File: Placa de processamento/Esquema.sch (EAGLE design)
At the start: 14 parts

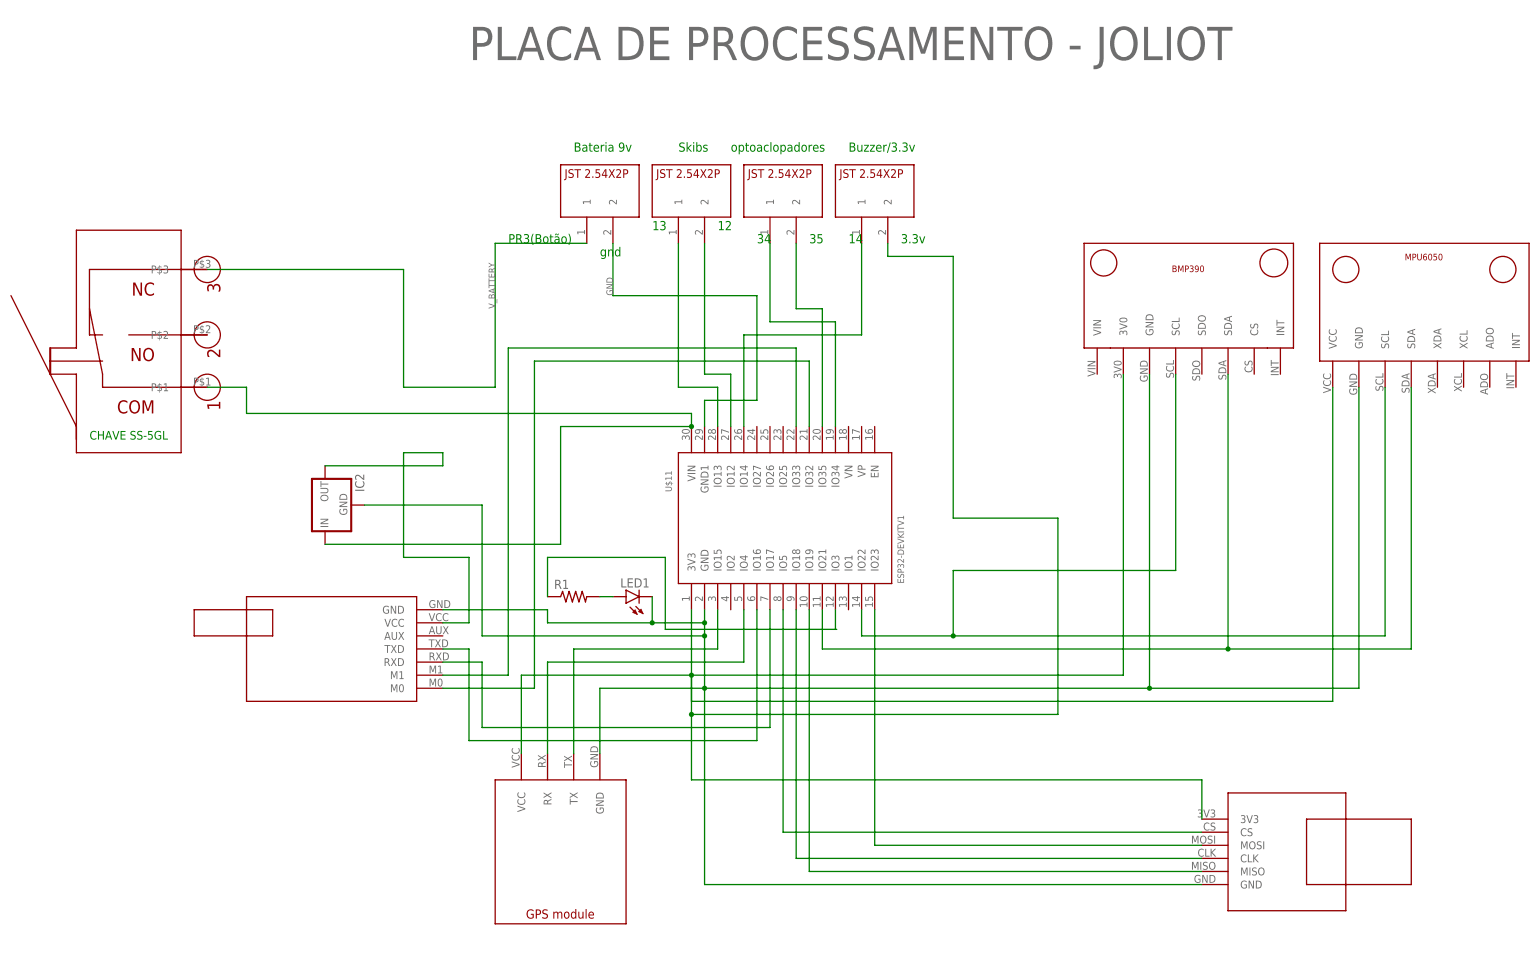
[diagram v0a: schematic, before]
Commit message: Coisas
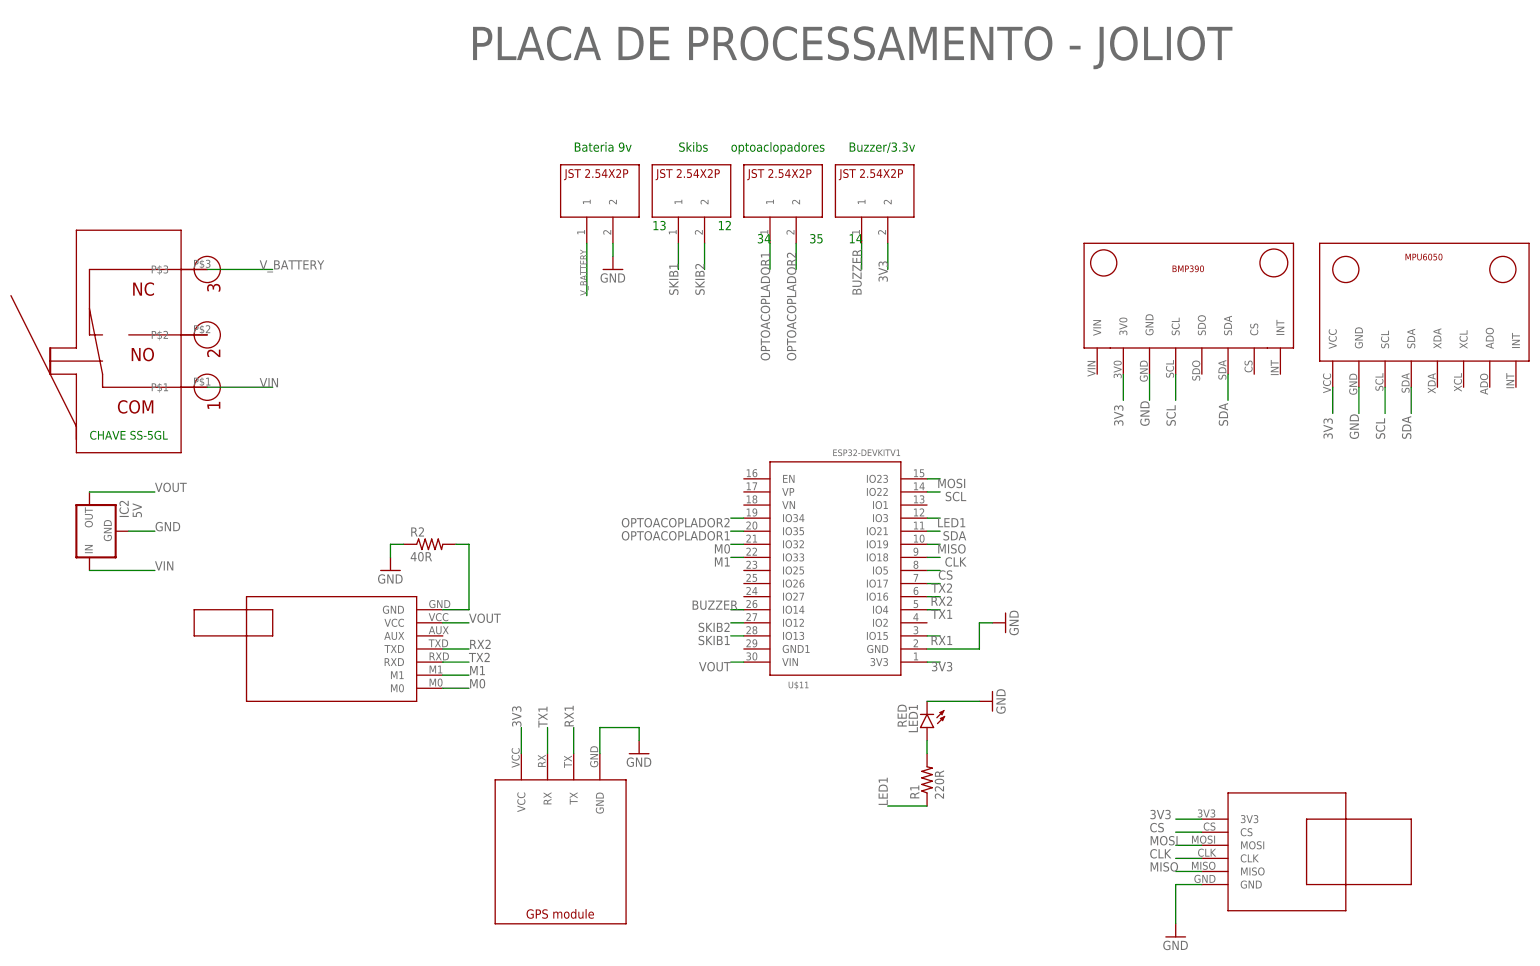
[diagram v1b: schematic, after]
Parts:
- added R2: 40R, rcl:R-US_0309/12
- IC2: value (none) -> 5V
- LED1: value (none) -> RED
- R1: value (none) -> 220R
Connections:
- net N$1 renamed SDA
- net N$10 renamed M1
- net N$11 renamed M0
- net N$13 renamed CS
- net N$14 renamed MOSI
- net N$15 renamed CLK
- net N$16 renamed MISO
- net N$17 renamed LED1
- net N$19 renamed SKIB1
- net N$2 renamed SCL
- net N$20 renamed SKIB2
- net N$21 renamed BUZZER
- net N$3 renamed 3V3
- net N$5 renamed TX1
- net N$6 renamed RX1
- net N$8 renamed TX2
- net N$9 renamed RX2
- removed net N$12: IC2.OUT, U$2.VCC
- removed net N$22: U$11.IO34, U$5.1
- removed net N$23: U$11.IO35, U$5.2
- new net OPTOACOPLADOR1: U$11.IO35, U$5.1
- new net OPTOACOPLADOR2: U$11.IO34, U$5.2
- new net VIN: IC2.IN, U$12.P$1
- new net VOUT: IC2.OUT, U$11.VIN, U$2.VCC
- net GND: now also R2.1; no longer U$11.GND1, U$2.GND
- net N$7: now also R2.2, U$2.GND; no longer IC2.IN, U$11.VIN, U$12.P$1
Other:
- note removed: "3.3v"
- note removed: "PR3(Botão)"
- note removed: "gnd"
- moved on the sheet: IC2, LED1, R1, U$11
